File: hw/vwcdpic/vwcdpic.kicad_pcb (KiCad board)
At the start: 2 copper layers, 14.6 x 13.1 mm, 12 parts, among them U1 PIC12F629, U2 LM78L05ACZ, U3 MC78L05ACH

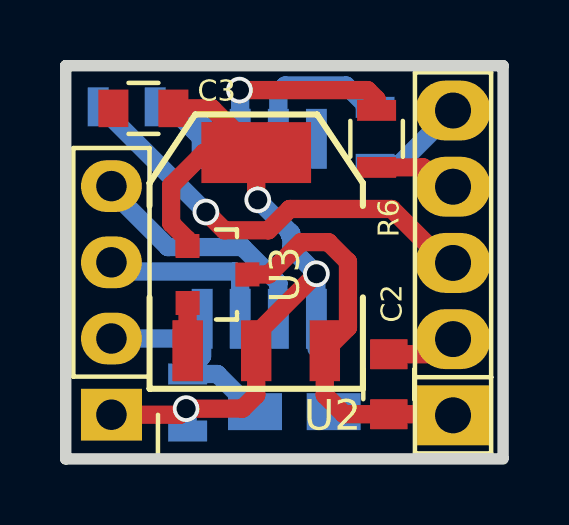
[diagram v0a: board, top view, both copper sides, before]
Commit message: update, new schematics file
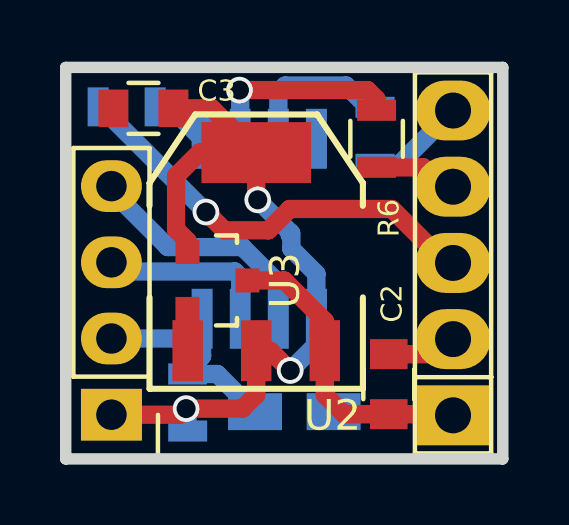
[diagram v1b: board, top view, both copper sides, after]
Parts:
- moved U3 0.20 mm to (142.8, 121.5)
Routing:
- net POWER_CTL: track 13.5 -> 10.3 mm
- net GND: track 3.99 -> 2.41 mm
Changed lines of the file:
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@@
     (links 26)
     (no_connects 0)
-    (area 137.579099 114.160299 152.539701 127.647701)
+    (area 137.579099 114.216179 152.529541 127.647701)
     (thickness 1.6002)
     (drawings 6)
-    (tracks 96)
+    (tracks 94)
     (zones 0)
     (modules 12)
@@
   (layers
     (0 Front signal)
-    (31 Back signal hide)
+    (31 Back signal)
     (32 B.Adhes user hide)
     (33 F.Adhes user hide)
@@
     (mod_text_size 1.524 1.524)
     (mod_text_width 0.3048)
-    (pad_size 2 2.5)
-    (pad_drill 1.2)
+    (pad_size 1.016 2.032)
+    (pad_drill 0)
     (pad_to_mask_clearance 0.254)
     (aux_axis_origin 0 0)
-    (visible_elements FFFEDBBF)
+    (visible_elements FFFEDFBF)
     (pcbplotparams
       (layerselection 0x0100f_80000001)
@@
       (at (xyz 0 0 0))
       (scale (xyz 1 1 1))
-      (rotate (xyz 0 0 0))
+      (rotate (xyz 0 0 90))
     )
   )
@@
     (pad 4 thru_hole oval (at 0 7.62 180) (size 2.032 1.7272) (drill 1.016) (layers *.Cu *.Mask F.SilkS)
       (net 10 ARCHOS))
-    (model Pin_Headers.3dshapes/Pin_Header_Straight_1x04.wrl
-      (at (xyz 0 -0.15 0))
-      (scale (xyz 1 1 1))
-      (rotate (xyz 0 0 90))
-    )
   )
   (module Capacitors_Tantalum_SMD:TantalC_SizeA_EIA-3216_Reflow (layer Back)
@@
     (model /home/nail/src/kicad/KiCad/3d_models/ab2_sot/AB2_SOT223.wrl
       (at (xyz 0 0 0))
-      (scale (xyz 1 1 1))
+      (scale (xyz 0 0 0))
       (rotate (xyz 0 0 0))
     )
   )
   (module Housings_SOT-23_SOT-143_TSOT-6:SOT-23 (layer Front)
-    (at 142.82928 121.3104 270)
+    (at 142.82928 121.50852 270)
     (descr "SOT-23, Standard")
     (tags SOT-23)
@@
     (pad 3 smd rect (at 0 -0.99822 270) (size 0.8001 0.8001) (layers Front F.Paste F.Mask)
       (net 3 POWER_CTL))
-    (model Housings_SOT-23_SOT-143_TSOT-6.3dshapes/SOT-23.wrl
-      (at (xyz 0 0 0))
-      (scale (xyz 1 1 1))
-      (rotate (xyz 0 0 0))
-    )
-  )
+    (model TO_SOT_Packages_SMD.3dshapes/SOT-23.wrl
+      (at (xyz 0 0 0))
+      (scale (xyz 1 1 1))
+      (rotate (xyz 0 0 0))
+    )
+  )
+  (gr_line (start 152.33904 127.4572) (end 137.7696 127.4572) (angle 90) (layer Edge.Cuts) (width 0.381))
+  (gr_line (start 152.33904 114.40668) (end 152.33904 127.4572) (angle 90) (layer Edge.Cuts) (width 0.381))
+  (gr_line (start 137.7696 114.40668) (end 152.33904 114.40668) (angle 90) (layer Edge.Cuts) (width 0.381))
+  (gr_line (start 137.7696 127.4572) (end 137.7696 114.40668) (angle 90) (layer Edge.Cuts) (width 0.381))
   (dimension 13.0556 (width 0.3048) (layer Dwgs.User)
     (gr_text "13.056 mm" (at 155.7528 120.9294 270) (layer Dwgs.User)
@@
     (arrow2b (pts (xy 137.7696 111.8108) (xy 138.896104 111.224379)))
   )
-  (gr_line (start 137.7696 127.4572) (end 137.7696 114.3508) (angle 90) (layer Edge.Cuts) (width 0.381))
-  (gr_line (start 152.3492 127.4572) (end 137.7696 127.4572) (angle 90) (layer Edge.Cuts) (width 0.381))
-  (gr_line (start 137.7696 114.3508) (end 152.3492 114.3508) (angle 90) (layer Edge.Cuts) (width 0.381))
-  (gr_line (start 152.3492 114.3508) (end 152.3492 127.4064) (angle 90) (layer Edge.Cuts) (width 0.381))
-  (segment (start 141.82852 120.3604) (end 141.82852 120.14708) (width 0.6096) (layer Front) (net 1) (status C00000))
-  (segment (start 141.82852 120.14708) (end 141.28496 119.60352) (width 0.6096) (layer Front) (net 1) (status 400000))
-  (segment (start 141.28496 119.60352) (end 141.28496 118.34368) (width 0.6096) (layer Front) (net 1))
-  (segment (start 141.28496 118.34368) (end 142.38224 117.2464) (width 0.6096) (layer Front) (net 1) (status 800000))
-  (segment (start 142.38224 117.2464) (end 144.1196 117.2464) (width 0.6096) (layer Front) (net 1) (status C00000))
+  (segment (start 141.82852 120.55852) (end 141.82852 120.18772) (width 0.6096) (layer Front) (net 1))
+  (segment (start 141.82852 120.18772) (end 141.44752 119.80672) (width 0.6096) (layer Front) (net 1))
+  (segment (start 141.44752 119.80672) (end 141.44752 118.02872) (width 0.6096) (layer Front) (net 1))
+  (segment (start 141.44752 118.02872) (end 142.22984 117.2464) (width 0.6096) (layer Front) (net 1))
+  (segment (start 142.22984 117.2464) (end 144.1196 117.2464) (width 0.6096) (layer Front) (net 1))
+  (segment (start 144.1196 123.8504) (end 144.59204 123.8504) (width 0.6096) (layer Front) (net 1))
+  (segment (start 144.59204 123.8504) (end 145.25244 124.5108) (width 0.6096) (layer Front) (net 1))
+  (segment (start 145.25244 124.5108) (end 146.1262 123.63704) (width 0.6096) (layer Back) (net 1))
+  (via (at 145.25244 124.5108) (size 0.889) (drill 0.635) (layers Front Back) (net 1))
+  (segment (start 146.1262 123.63704) (end 146.1262 122.7864) (width 0.6096) (layer Back) (net 1))
   (segment (start 141.3604 115.7732) (end 142.6464 115.7732) (width 0.6096) (layer Front) (net 1))
   (segment (start 142.6464 115.7732) (end 144.1196 117.2464) (width 0.6096) (layer Front) (net 1))
   (segment (start 146.1262 122.7864) (end 146.1262 121.285) (width 0.6096) (layer Back) (net 1))
-  (via (at 146.1262 121.285) (size 0.889) (drill 0.635) (layers Front Back) (net 1))
-  (segment (start 146.1262 121.285) (end 144.1196 123.2916) (width 0.6096) (layer Front) (net 1))
   (segment (start 144.1196 123.2916) (end 144.1196 123.8504) (width 0.6096) (layer Front) (net 1))
-  (segment (start 146.1262 123.7742) (end 146.1262 122.7864) (width 0.6096) (layer Back) (net 1))
   (segment (start 145.2372 119.9896) (end 145.2372 119.888) (width 0.6096) (layer Back) (net 1))
   (segment (start 145.288 119.9388) (end 145.2372 119.9896) (width 0.6096) (layer Back) (net 1))
@@
   (via (at 141.7828 125.7808) (size 0.889) (drill 0.635) (layers Front Back) (net 1))
   (segment (start 141.5796 125.984) (end 141.7828 125.7808) (width 0.6096) (layer Front) (net 1))
-  (segment (start 141.82852 122.2604) (end 141.82852 123.84532) (width 0.6096) (layer Front) (net 2) (status C00000))
-  (segment (start 141.82852 123.84532) (end 141.8336 123.8504) (width 0.6096) (layer Front) (net 2) (status C00000))
+  (segment (start 141.82852 123.84532) (end 141.8336 123.8504) (width 0.6096) (layer Front) (net 2))
   (segment (start 148.5392 123.968) (end 150.17674 123.968) (width 0.6096) (layer Front) (net 2))
   (segment (start 150.17674 123.968) (end 150.68042 123.46432) (width 0.6096) (layer Front) (net 2))
   (segment (start 141.8336 123.7996) (end 141.8336 123.8504) (width 0.6096) (layer Front) (net 2))
-  (segment (start 143.8275 121.3104) (end 144.53616 121.3104) (width 0.6096) (layer Front) (net 3) (status 400000))
-  (segment (start 147.17776 123.07824) (end 146.4056 123.8504) (width 0.6096) (layer Front) (net 3) (status 800000))
-  (segment (start 147.17776 120.88368) (end 147.17776 123.07824) (width 0.6096) (layer Front) (net 3))
-  (segment (start 146.52752 120.23344) (end 147.17776 120.88368) (width 0.6096) (layer Front) (net 3))
-  (segment (start 145.61312 120.23344) (end 146.52752 120.23344) (width 0.6096) (layer Front) (net 3))
-  (segment (start 144.53616 121.3104) (end 145.61312 120.23344) (width 0.6096) (layer Front) (net 3))
+  (segment (start 146.4056 123.8504) (end 146.4056 122.8598) (width 0.6096) (layer Front) (net 3))
+  (segment (start 146.4056 122.8598) (end 145.05432 121.50852) (width 0.6096) (layer Front) (net 3))
+  (segment (start 145.05432 121.50852) (end 143.8275 121.50852) (width 0.6096) (layer Front) (net 3))
   (segment (start 148.5392 125.968) (end 150.6441 125.968) (width 0.6096) (layer Front) (net 3))
   (segment (start 150.6441 125.968) (end 150.68042 126.00432) (width 0.6096) (layer Front) (net 3))
